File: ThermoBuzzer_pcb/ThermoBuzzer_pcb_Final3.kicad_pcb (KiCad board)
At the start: 2 copper layers, 60 x 60 mm, 13 parts, among them SW2 SW_Push

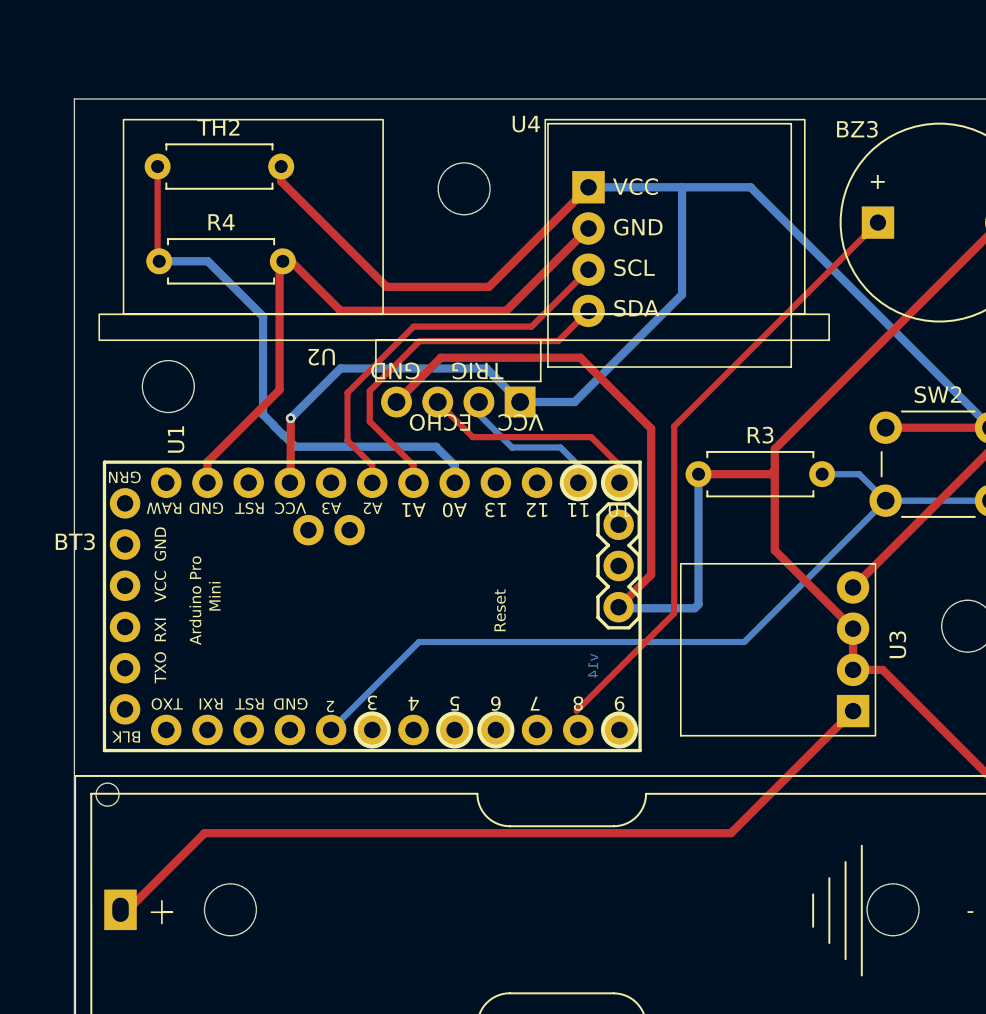
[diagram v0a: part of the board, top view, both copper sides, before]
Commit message: 4.28
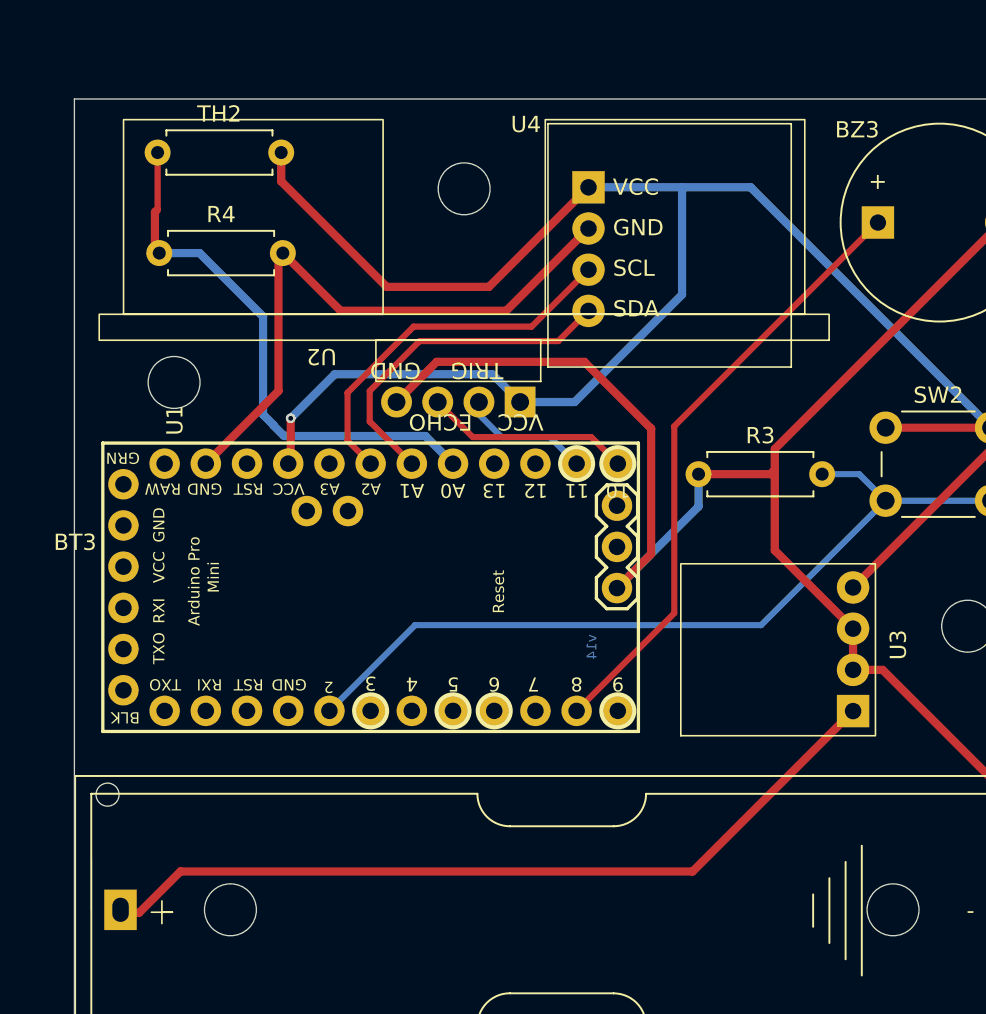
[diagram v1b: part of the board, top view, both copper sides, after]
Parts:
- moved U1 1.18 mm to (127.6, 106.2)
- moved TH2 0.86 mm to (99.1, 71.9)
- moved R4 0.51 mm to (99.2, 78.1)
- moved ? 0.44 mm to (100.1, 86.1)
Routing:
- net GND: track 103.7 -> 98.4 mm
- net Net-(U1-11): track 9.26 -> 8.04 mm
- net Net-(U1-A2): track 24.2 -> 23.0 mm
- net Net-(U1-A1): track 22.3 -> 21.1 mm
- net Net-(U1-10): track 13.9 -> 12.7 mm
- net +3.3V: track 115.5 -> 115.0 mm
- net Net-(U1-A0): track 33.9 -> 33.4 mm
